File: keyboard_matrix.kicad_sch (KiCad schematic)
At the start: 85 parts

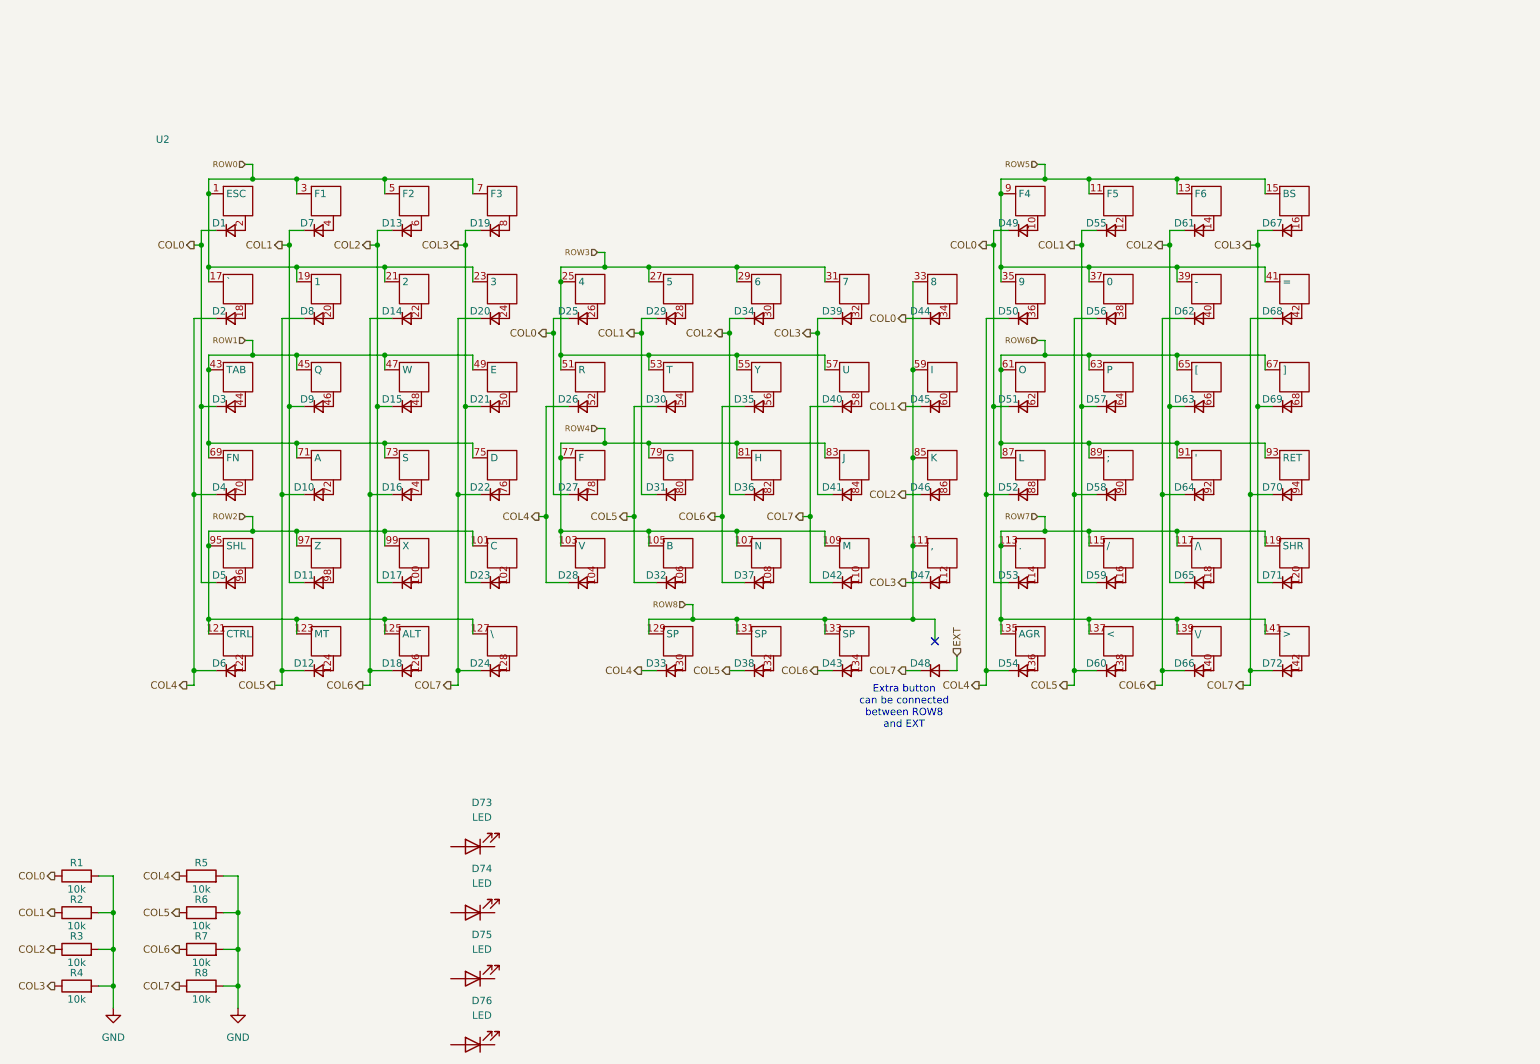
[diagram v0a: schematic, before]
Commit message: Relabeling of ESP32-C6 GPIO, route signals to expansion header for testing
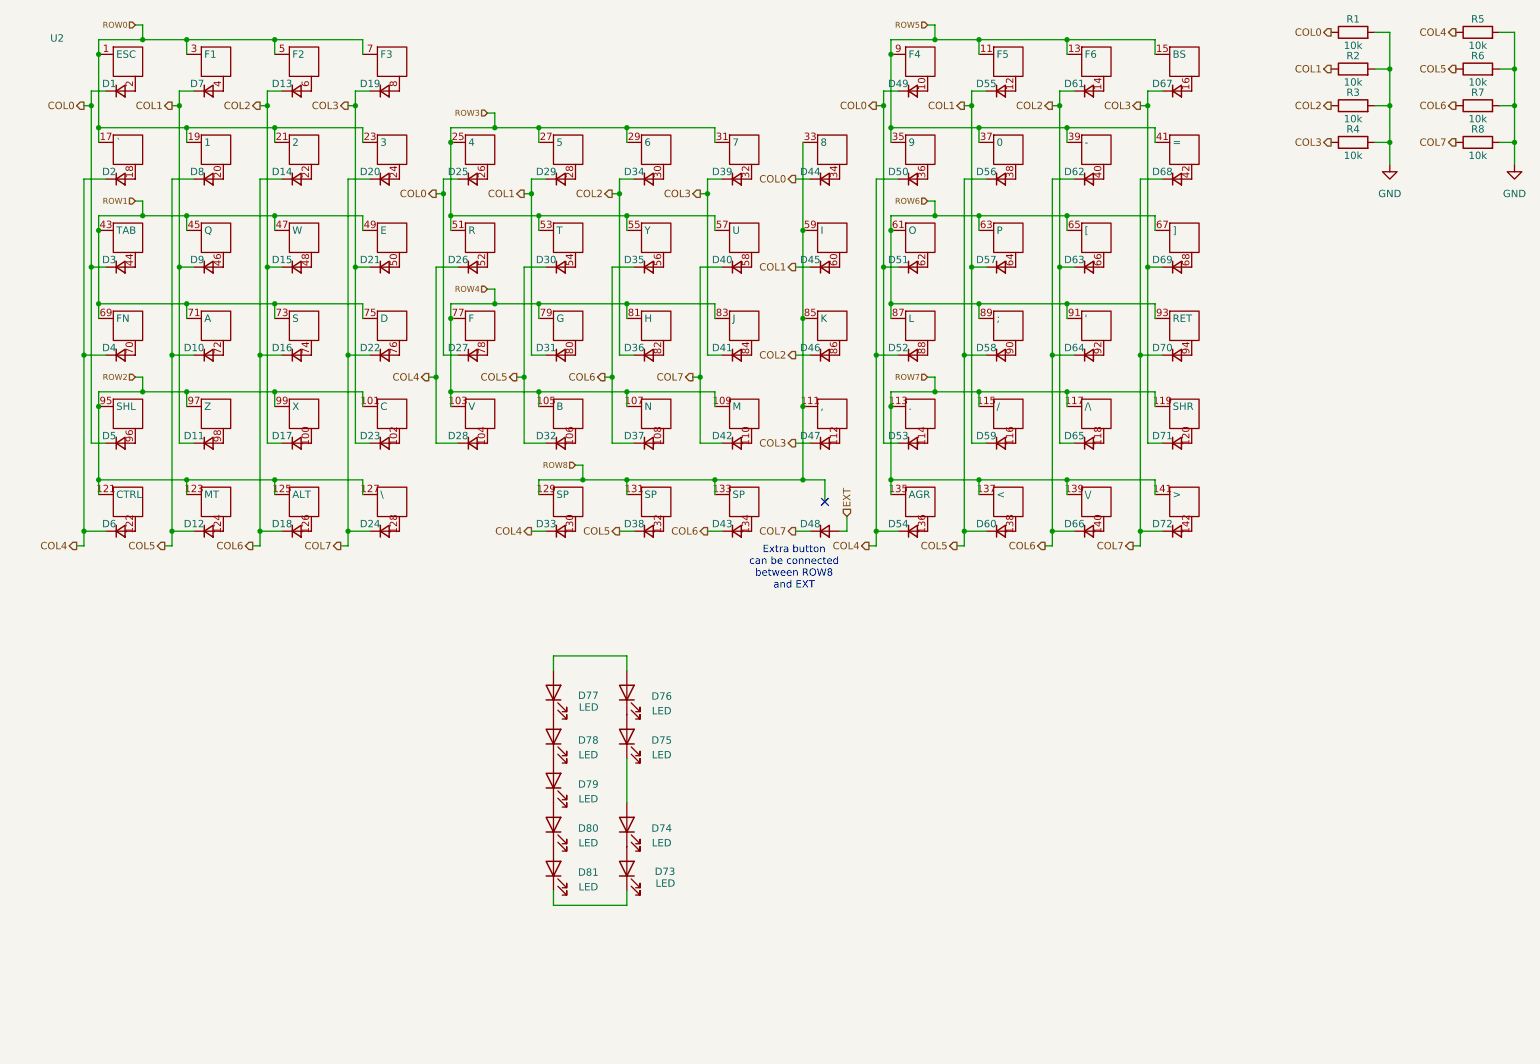
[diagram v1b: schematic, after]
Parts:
- added D77, D78, D79, D80, D81: LED, badgeteam:LTW-010DCG-SR-G, symbol Device:LED
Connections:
- net at D75.1 (K): now also D74.2 (A)
- net at D75.2 (A): now also D76.1 (K)
- net at D73.1 (K): now also D81.1 (K)
- net at D73.2 (A): now also D74.1 (K)
- net at D76.2 (A): now also D77.2 (A)
- new net: D80.1 (K), D81.2 (A)
- new net: D79.1 (K), D80.2 (A)
- new net: D77.1 (K), D78.2 (A)
- new net: D78.1 (K), D79.2 (A)
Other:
- moved on the sheet: D1, D10, D11, D12, D13, D14, D15, D16, D17, D18, D19, D2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
